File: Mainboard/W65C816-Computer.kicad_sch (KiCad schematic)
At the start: 113 parts, among them J1 ADDR_DATA_DBG, J2 CTRL_BANK_DBG, J3 CPU_MISC_DBG, J4 POWER_IN_HEADER_8A, J5 DAUGHTER_PWR_AUX, J6 ISA16_DAUGHTER_BUS, J7 PWR_LED_HEADER, J8 RESET_HEADER, Q1 P-MOSFET_REV_PROT_TO220, SW2 NMI, SW3 MAIN_PWR_SW_EXT, U1 W65C816S6PG-14, U10 SN74HC04N, U11 SN74HC08N, U12 SN74HC139N, U16 SN74HC245N, U17 SN74HC32N, U18 SN74HC04N, U2 SN74HC573N, U20 AS6C4008-55PCN, U21 AS6C4008-55PCN, U22 AS6C4008-55PCN, U23 AS6C4008-55PCN, U24 AS6C4008-55PCN, U25 AS6C4008-55PCN, U26 AS6C4008-55PCN, U27 AS6C4008-55PCN, U3 SN74HC245N, U30 SST39VF040-70-4I-NHE, U4 MCP130-315D, U5 SN74HC14N, U6 SN74HC138N, U7 SN74HC138N, U8 SN74HC138N, U9 SN74HC00N, X1 ECS-P143X-8.000-BN

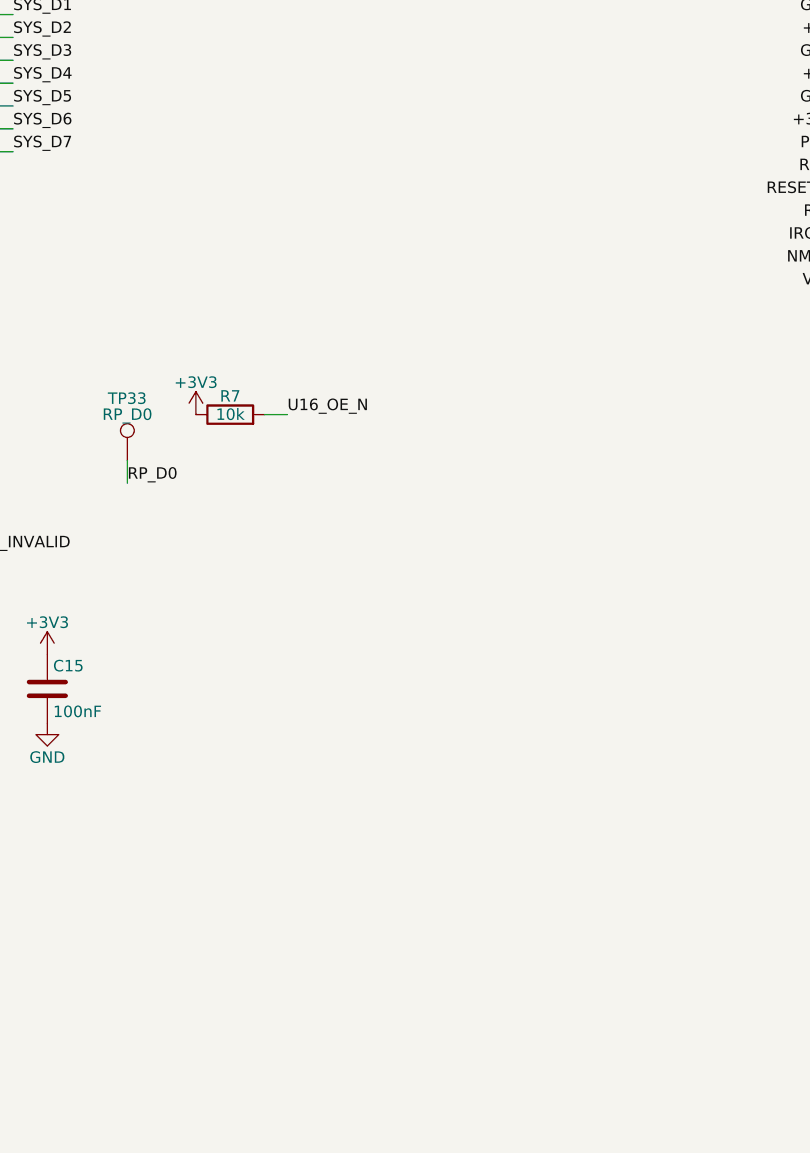
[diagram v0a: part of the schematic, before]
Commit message: Place and terminate unused U18 gates
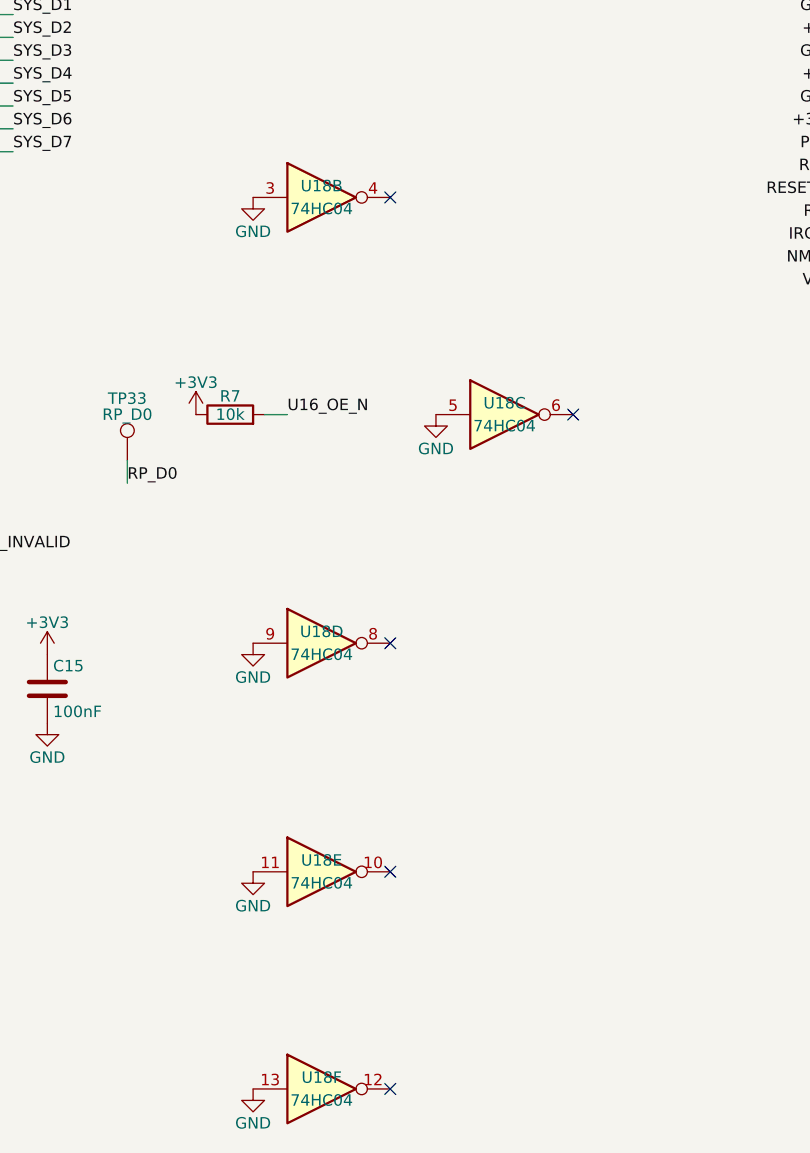
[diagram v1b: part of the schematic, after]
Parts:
- added unit 3 of U18
- added unit 5 of U18
- added unit 6 of U18
- added unit 4 of U18
- added unit 2 of U18
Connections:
- net GND: now also U18.11, U18.13, U18.3, U18.5, U18.9
- no-connect marks 50 -> 55
